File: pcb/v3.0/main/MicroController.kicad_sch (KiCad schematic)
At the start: 35 parts, among them J1 Magnet, J14 PH, J2 PH, SW1 RESET, SW2 USER, U2 STM32G431CB, U3 MCP2562-E-SN, Y1 XRCGB16M000FXN02R0

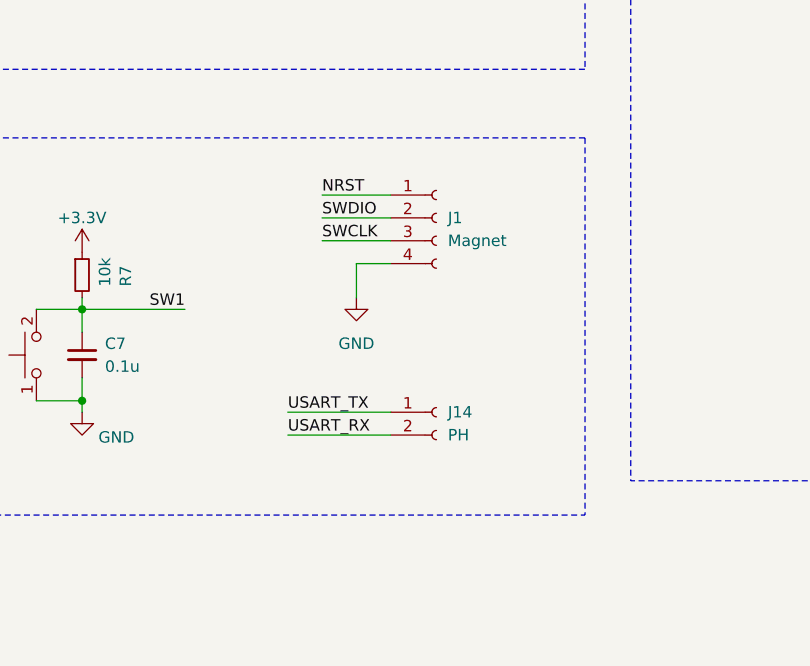
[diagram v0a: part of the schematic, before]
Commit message: chore: add pdf
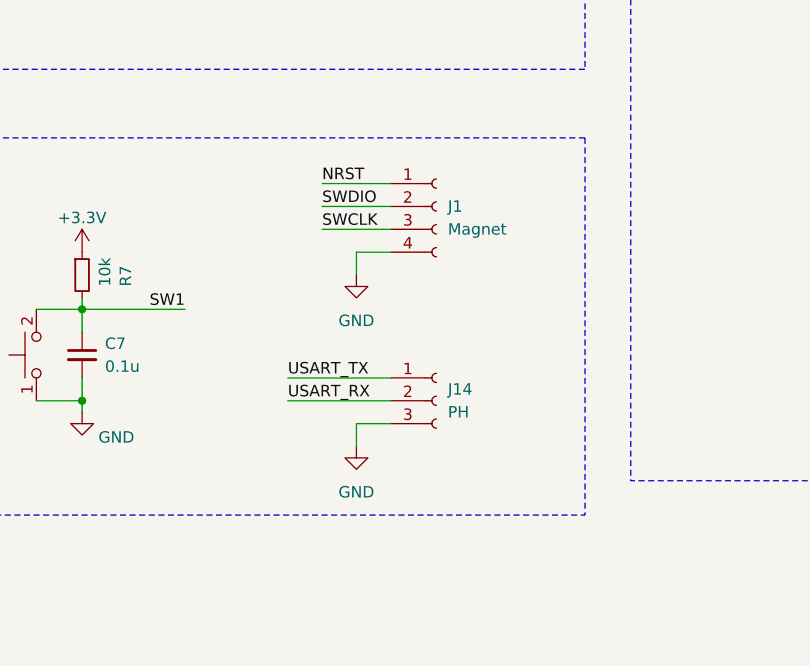
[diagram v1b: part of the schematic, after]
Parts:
- J14: footprint Connector_JST:JST_PH_S2B-PH-K_1x02_P2.00mm_Horizontal -> Connector_JST:JST_PH_S3B-PH-K_1x03_P2.00mm_Horizontal; symbol Connector:Conn_01x02_Socket -> Connector:Conn_01x03_Socket
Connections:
- net GND: now also J14.3 (Pin_3)
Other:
- moved on the sheet: J1
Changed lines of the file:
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@@
 	(wire
 		(pts
-			(xy 139.7 157.48) (xy 151.13 157.48)
-		)
-		(stroke
-			(width 0)
-			(type default)
-		)
-	)
-	(wire
-		(pts
 			(xy 22.86 180.34) (xy 25.4 180.34)
 		)
@@
 	(wire
 		(pts
-			(xy 151.13 138.43) (xy 147.32 138.43)
+			(xy 151.13 137.16) (xy 147.32 137.16)
 		)
 		(stroke
@@
 	(wire
 		(pts
-			(xy 143.51 130.81) (xy 151.13 130.81)
+			(xy 143.51 129.54) (xy 151.13 129.54)
 		)
 		(stroke
@@
 	(wire
 		(pts
-			(xy 143.51 133.35) (xy 151.13 133.35)
+			(xy 143.51 132.08) (xy 151.13 132.08)
 		)
 		(stroke
@@
 	(wire
 		(pts
+			(xy 147.32 156.21) (xy 151.13 156.21)
+		)
+		(stroke
+			(width 0)
+			(type default)
+		)
+	)
+	(wire
+		(pts
 			(xy 21.59 52.07) (xy 21.59 55.88)
 		)
@@
 	(wire
 		(pts
+			(xy 147.32 158.75) (xy 147.32 156.21)
+		)
+		(stroke
+			(width 0)
+			(type default)
+		)
+	)
+	(wire
+		(pts
 			(xy 92.71 143.51) (xy 90.17 143.51)
 		)
@@
 	(wire
 		(pts
-			(xy 143.51 135.89) (xy 151.13 135.89)
+			(xy 143.51 134.62) (xy 151.13 134.62)
 		)
 		(stroke
@@
 	(wire
 		(pts
-			(xy 147.32 138.43) (xy 147.32 142.24)
+			(xy 147.32 137.16) (xy 147.32 139.7)
 		)
 		(stroke
@@
 	(wire
 		(pts
-			(xy 91.44 81.28) (xy 104.14 81.28)
+			(xy 139.7 151.13) (xy 151.13 151.13)
 		)
 		(stroke
@@
 	(wire
 		(pts
-			(xy 217.17 107.95) (xy 217.17 109.22)
+			(xy 91.44 81.28) (xy 104.14 81.28)
 		)
 		(stroke
@@
 	(wire
 		(pts
-			(xy 139.7 154.94) (xy 151.13 154.94)
+			(xy 217.17 107.95) (xy 217.17 109.22)
 		)
 		(stroke
@@
 	(wire
 		(pts
+			(xy 139.7 153.67) (xy 151.13 153.67)
+		)
+		(stroke
+			(width 0)
+			(type default)
+		)
+	)
+	(wire
+		(pts
 			(xy 96.52 26.67) (xy 96.52 25.4)
 		)
@@
 	)
 	(label "USART_TX"
-		(at 139.7 154.94 0)
+		(at 139.7 151.13 0)
 		(fields_autoplaced yes)
 		(effects
@@
 	)
 	(label "NRST"
-		(at 143.51 130.81 0)
+		(at 143.51 129.54 0)
 		(fields_autoplaced yes)
 		(effects
@@
 	)
 	(label "SWCLK"
-		(at 143.51 135.89 0)
+		(at 143.51 134.62 0)
 		(fields_autoplaced yes)
 		(effects
@@
 	)
 	(label "SWDIO"
-		(at 143.51 133.35 0)
+		(at 143.51 132.08 0)
 		(fields_autoplaced yes)
 		(effects
@@
 	)
 	(label "USART_RX"
-		(at 139.7 157.48 0)
+		(at 139.7 153.67 0)
 		(fields_autoplaced yes)
 		(effects
@@
 	)
 	(symbol
-		(lib_id "Connector:Conn_01x02_Socket")
-		(at 156.21 154.94 0)
+		(lib_id "Connector:Conn_01x03_Socket")
+		(at 156.21 153.67 0)
 		(unit 1)
 		(exclude_from_sim no)
@@
 		(fields_autoplaced yes)
 		(property "Reference" "J14"
-			(at 157.48 154.9399 0)
+			(at 157.48 152.3999 0)
 			(effects
 				(font
@@
 		)
 		(property "Value" "PH"
-			(at 157.48 157.4799 0)
+			(at 157.48 154.9399 0)
 			(effects
 				(font
@@
 			)
 		)
-		(property "Footprint" "Connector_JST:JST_PH_S2B-PH-K_1x02_P2.00mm_Horizontal"
-			(at 156.21 154.94 0)
+		(property "Footprint" "Connector_JST:JST_PH_S3B-PH-K_1x03_P2.00mm_Horizontal"
+			(at 156.21 153.67 0)
 			(effects
 				(font
@@
 		)
 		(property "Datasheet" "~"
-			(at 156.21 154.94 0)
+			(at 156.21 153.67 0)
 			(effects
 				(font
@@
 			)
 		)
-		(property "Description" "Generic connector, single row, 01x02, script generated"
-			(at 156.21 154.94 0)
+		(property "Description" "Generic connector, single row, 01x03, script generated"
+			(at 156.21 153.67 0)
 			(effects
 				(font
@@
 		(pin "1"
 		)
+		(pin "3"
+		)
 		(instances
 			(project ""
@@
 	)
 	(symbol
+		(lib_id "power:GND")
+		(at 147.32 158.75 0)
+		(unit 1)
+		(exclude_from_sim no)
+		(in_bom yes)
+		(on_board yes)
+		(dnp no)
+		(fields_autoplaced yes)
+		(property "Reference" "#PWR01"
+			(at 147.32 165.1 0)
+			(effects
+				(font
+					(size 1.27 1.27)
+				)
+				(hide yes)
+			)
+		)
+		(property "Value" "GND"
+			(at 147.32 163.83 0)
+			(effects
+				(font
+					(size 1.27 1.27)
+				)
+			)
+		)
+		(property "Footprint" ""
+			(at 147.32 158.75 0)
+			(effects
+				(font
+					(size 1.27 1.27)
+				)
+				(hide yes)
+			)
+		)
+		(property "Datasheet" ""
+			(at 147.32 158.75 0)
+			(effects
+				(font
+					(size 1.27 1.27)
+				)
+				(hide yes)
+			)
+		)
+		(property "Description" ""
+			(at 147.32 158.75 0)
+			(effects
+				(font
+					(size 1.27 1.27)
+				)
+				(hide yes)
+			)
+		)
+		(pin "1"
+		)
+		(instances
+			(project "main"
+				(path "/1630ca0c-51c9-4aeb-9f5b-af64c3de63e1/890f87e9-49c3-4c63-bb8a-5b1e557cbd26"
+					(reference "#PWR01")
+					(unit 1)
+				)
+			)
+		)
+	)
+	(symbol
 		(lib_id "bldc_lib:STM32G431CB")
 		(at 62.23 69.85 0)
@@
 	(symbol
 		(lib_id "power:GND")
-		(at 147.32 142.24 0)
+		(at 147.32 139.7 0)
 		(unit 1)
 		(exclude_from_sim no)
@@
 		(fields_autoplaced yes)
 		(property "Reference" "#PWR035"
-			(at 147.32 148.59 0)
+			(at 147.32 146.05 0)
 			(effects
 				(font
@@
 		)
 		(property "Value" "GND"
-			(at 147.32 147.32 0)
+			(at 147.32 144.78 0)
 			(effects
 				(font
@@
 		)
 		(property "Footprint" ""
-			(at 147.32 142.24 0)
+			(at 147.32 139.7 0)
 			(effects
 				(font
@@
 		)
 		(property "Datasheet" ""
-			(at 147.32 142.24 0)
+			(at 147.32 139.7 0)
 			(effects
 				(font
@@
 		)
 		(property "Description" ""
-			(at 147.32 142.24 0)
+			(at 147.32 139.7 0)
 			(effects
 				(font
@@
 	(symbol
 		(lib_id "Connector:Conn_01x04_Female")
-		(at 156.21 133.35 0)
+		(at 156.21 132.08 0)
 		(unit 1)
 		(exclude_from_sim no)
@@
 		(fields_autoplaced yes)
 		(property "Reference" "J1"
-			(at 157.48 133.3499 0)
+			(at 157.48 132.0799 0)
 			(effects
 				(font
@@
 		)
 		(property "Value" "Magnet"
-			(at 157.48 135.8899 0)
+			(at 157.48 134.6199 0)
 			(effects
 				(font
@@
 		)
 		(property "Footprint" "Connector_PinSocket_2.54mm:PinSocket_1x04_P2.54mm_Vertical"
-			(at 156.21 133.35 0)
+			(at 156.21 132.08 0)
 			(effects
 				(font
@@
 		)
 		(property "Datasheet" "~"
-			(at 156.21 133.35 0)
+			(at 156.21 132.08 0)
 			(effects
 				(font
@@
 		)
 		(property "Description" ""
-			(at 156.21 133.35 0)
+			(at 156.21 132.08 0)
 			(effects
 				(font
